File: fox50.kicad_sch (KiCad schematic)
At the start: 112 parts

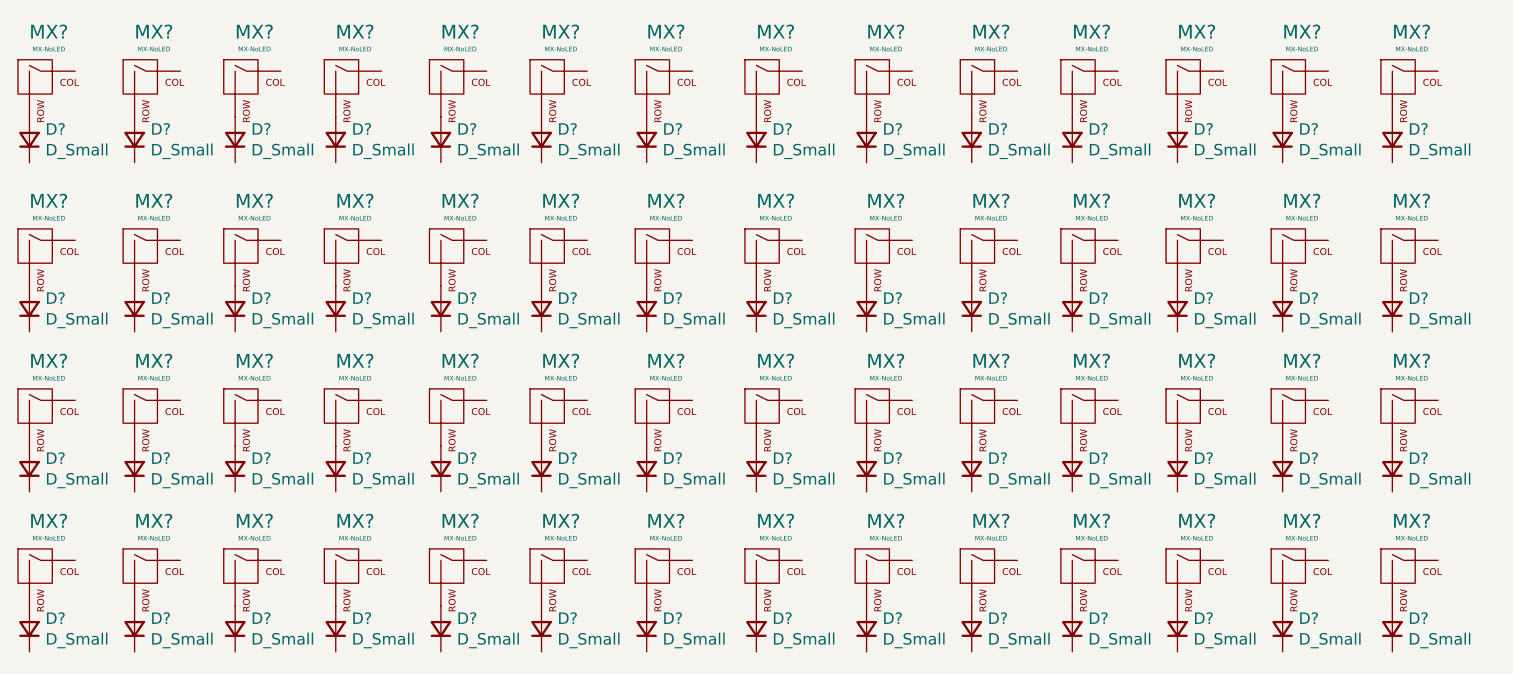
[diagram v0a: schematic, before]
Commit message: conexiones del eschema
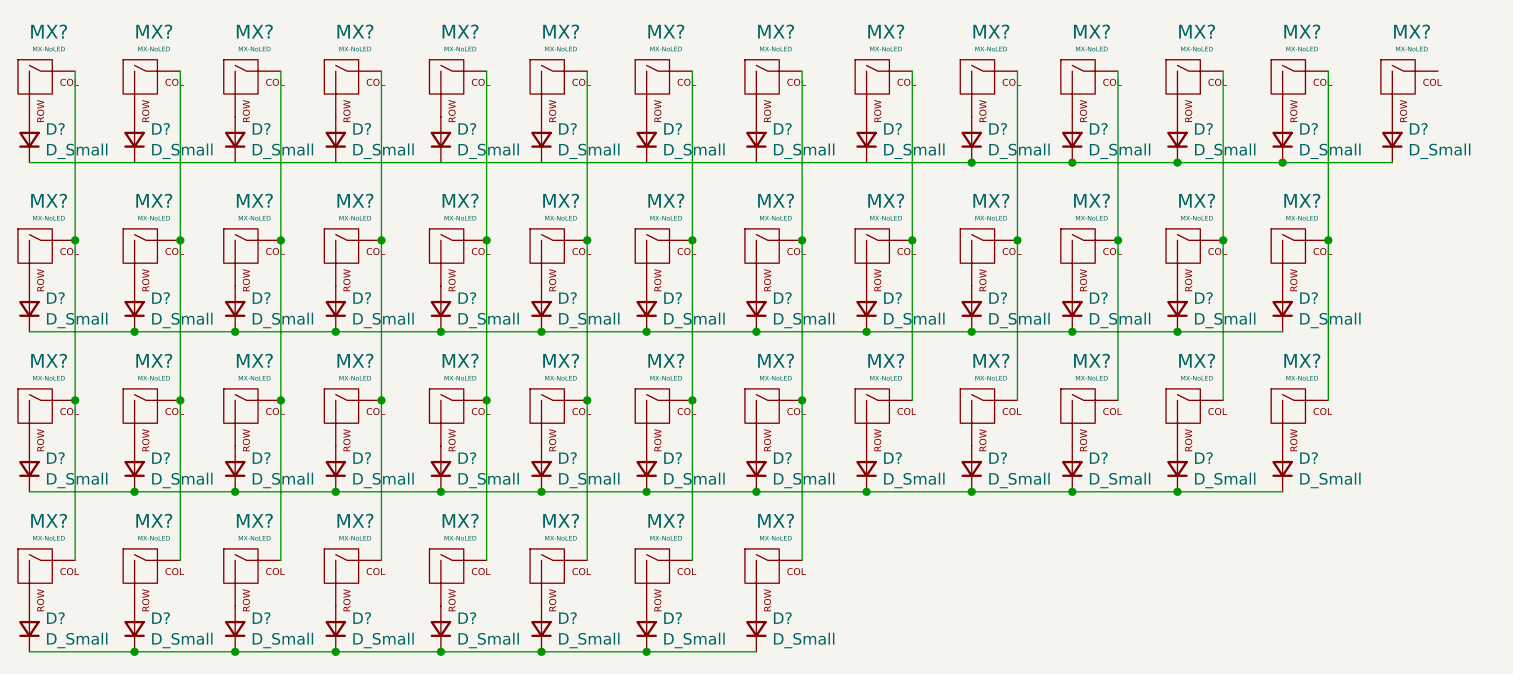
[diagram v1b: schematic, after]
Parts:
- removed D? (x8): D_Small, symbol res:D_Small
- removed MX? (x8): MX-NoLED, symbol mx:MX-NoLED
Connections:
- net at D?.1 (K): now also D?.1 (K), D?.1 (K), D?.1 (K), D?.1 (K), D?.1 (K), D?.1 (K), D?.1 (K), D?.1 (K), D?.1 (K), D?.1 (K), D?.1 (K), D?.1 (K) (x2)
- net at MX?.1 (COL): now also MX?.1 (COL), MX?.1 (COL), MX?.1 (COL) (x8)
- net at MX?.1 (COL): now also MX?.1 (COL), MX?.1 (COL) (x5)
- net at D?.1 (K): now also D?.1 (K), D?.1 (K), D?.1 (K), D?.1 (K), D?.1 (K), D?.1 (K), D?.1 (K)
- net at D?.1 (K): now also D?.1 (K), D?.1 (K), D?.1 (K), D?.1 (K), D?.1 (K)
